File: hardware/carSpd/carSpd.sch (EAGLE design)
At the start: 71 parts, among them IC1 DS3231/SO, IC2 CP2102, Q1 2n3904, U2 MP2307, U3 7805DT, U4 ATMEGA328P_TQFP, Y1 16MHZ, Y2 16mhz

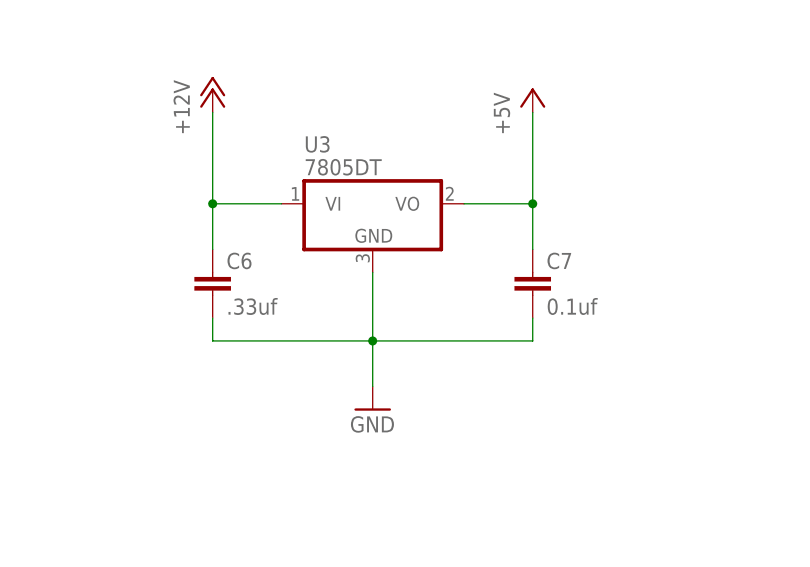
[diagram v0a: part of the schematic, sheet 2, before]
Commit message: Modified and added parts list
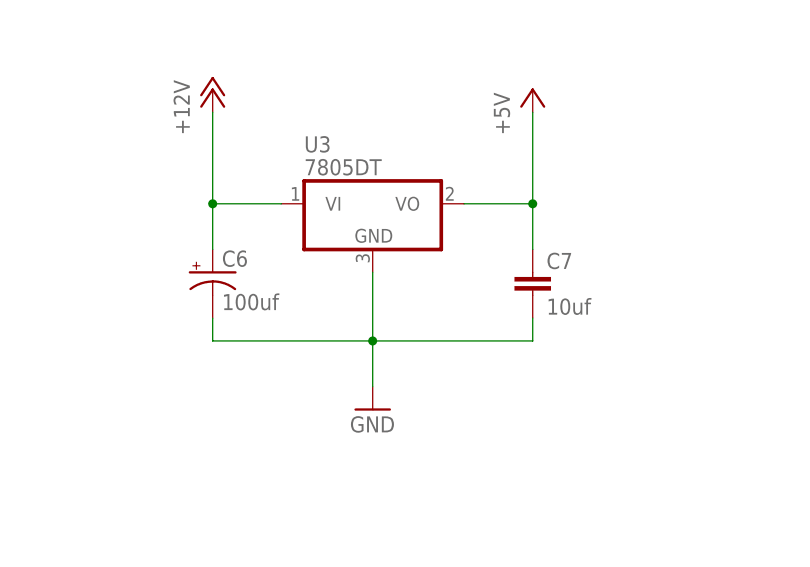
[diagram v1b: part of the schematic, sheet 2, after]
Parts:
- C6: value .33uf -> 100uf; device rcl:C-EUC0603K -> ELL-i-Passives:CPOLD
- C7: value 0.1uf -> 10uf
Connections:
- net +12V: now also C6.+; no longer C6.1
- net GND: now also C6.-; no longer C6.2
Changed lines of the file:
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@@
 <layer number="56" name="wert" color="7" fill="1" visible="yes" active="no"/>
 <layer number="57" name="tCAD" color="7" fill="1" visible="yes" active="no"/>
+<layer number="58" name="bCopper" color="7" fill="1" visible="no" active="no"/>
 <layer number="59" name="tCarbon" color="7" fill="1" visible="yes" active="no"/>
 <layer number="60" name="bCarbon" color="7" fill="1" visible="yes" active="no"/>
@@
 <layer number="250" name="Descript" color="7" fill="1" visible="no" active="no"/>
 <layer number="251" name="SMDround" color="7" fill="1" visible="no" active="no"/>
+<layer number="253" name="Extra" color="7" fill="1" visible="yes" active="yes"/>
 <layer number="254" name="cooling" color="7" fill="1" visible="no" active="yes"/>
 <layer number="255" name="HELP" color="7" fill="1" visible="yes" active="yes"/>
@@
 <part name="P+3" library="supply1" deviceset="+12V" device=""/>
 <part name="U3" library="adafruit" deviceset="78*" device="DT" technology="05"/>
-<part name="C6" library="rcl" deviceset="C-EU" device="C0603K" value=".33uf"/>
-<part name="C7" library="rcl" deviceset="C-EU" device="C0603K" value="0.1uf"/>
+<part name="C7" library="rcl" deviceset="C-EU" device="C0603K" value="10uf"/>
 <part name="P+4" library="supply1" deviceset="+12V" device=""/>
 <part name="P+5" library="supply1" deviceset="+5V" device=""/>
@@
 <part name="FRAME5" library="frames" deviceset="A5L-LOC" device=""/>
 <part name="Y1" library="SparkFun-FreqCtrl" deviceset="RESONATOR" device="16MHZ" value="16MHZ"/>
+<part name="C6" library="ELL-i-Passives" deviceset="CPOL" device="D" value="100uf"/>
 </parts>
 <sheets>
@@
 <instances>
 <instance part="U3" gate="A1" x="208.28" y="129.54"/>
-<instance part="C6" gate="G$1" x="190.5" y="121.92"/>
 <instance part="C7" gate="G$1" x="226.06" y="121.92"/>
 <instance part="P+4" gate="1" x="190.5" y="142.24"/>
@@
 <instance part="P+3" gate="1" x="96.52" y="167.64"/>
 <instance part="FRAME4" gate="G$1" x="0" y="0"/>
+<instance part="C6" gate="G$1" x="190.5" y="121.92"/>
 </instances>
 <busses>
@@
 <net name="+12V" class="0">
 <segment>
-<pinref part="C6" gate="G$1" pin="1"/>
 <pinref part="P+4" gate="1" pin="+12V"/>
 <wire x1="190.5" y1="124.46" x2="190.5" y2="129.54" width="0.1524" layer="91"/>
@@
 <wire x1="190.5" y1="129.54" x2="198.12" y2="129.54" width="0.1524" layer="91"/>
 <junction x="190.5" y="129.54"/>
+<pinref part="C6" gate="G$1" pin="+"/>
 </segment>
 <segment>
@@
 <net name="GND" class="0">
 <segment>
-<pinref part="C6" gate="G$1" pin="2"/>
 <wire x1="190.5" y1="116.84" x2="190.5" y2="114.3" width="0.1524" layer="91"/>
 <pinref part="GND2" gate="1" pin="GND"/>
@@
 <wire x1="208.28" y1="114.3" x2="226.06" y2="114.3" width="0.1524" layer="91"/>
 <wire x1="226.06" y1="114.3" x2="226.06" y2="116.84" width="0.1524" layer="91"/>
-</segment>
-<segment>
+<pinref part="C6" gate="G$1" pin="-"/>
+</segment>
+<segment>
